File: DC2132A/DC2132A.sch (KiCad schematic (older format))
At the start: 5 parts, among them U3 LT8612

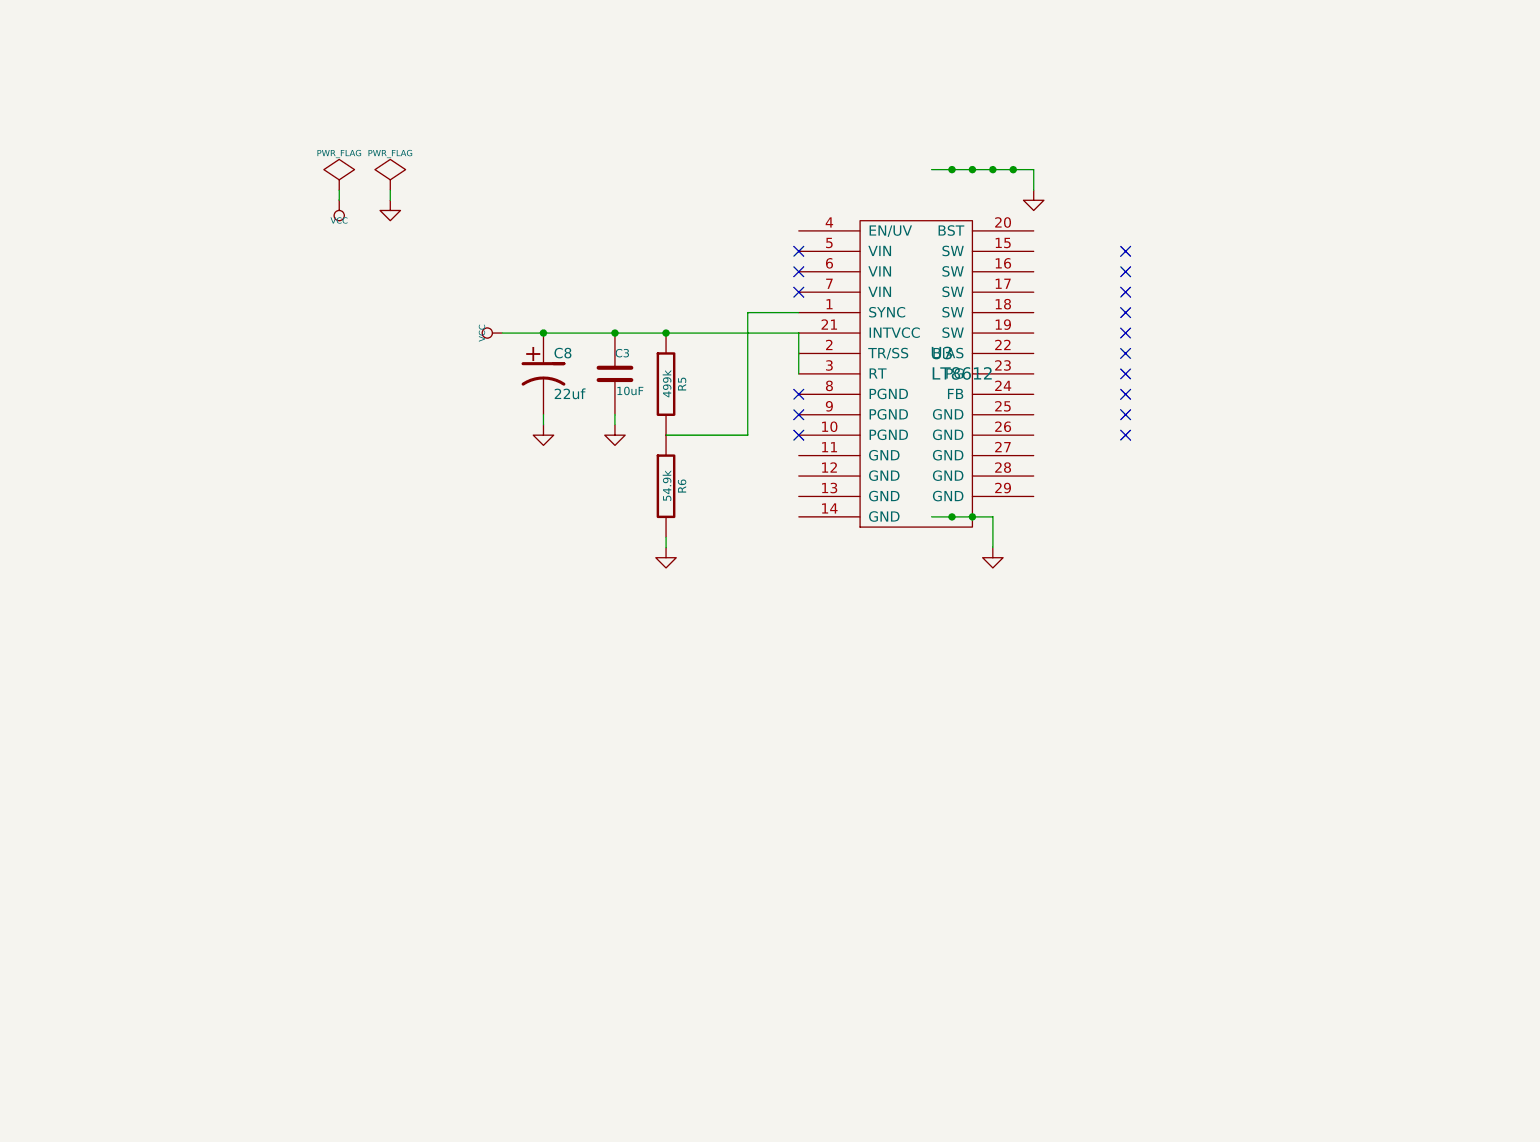
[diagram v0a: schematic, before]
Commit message: new kicad version
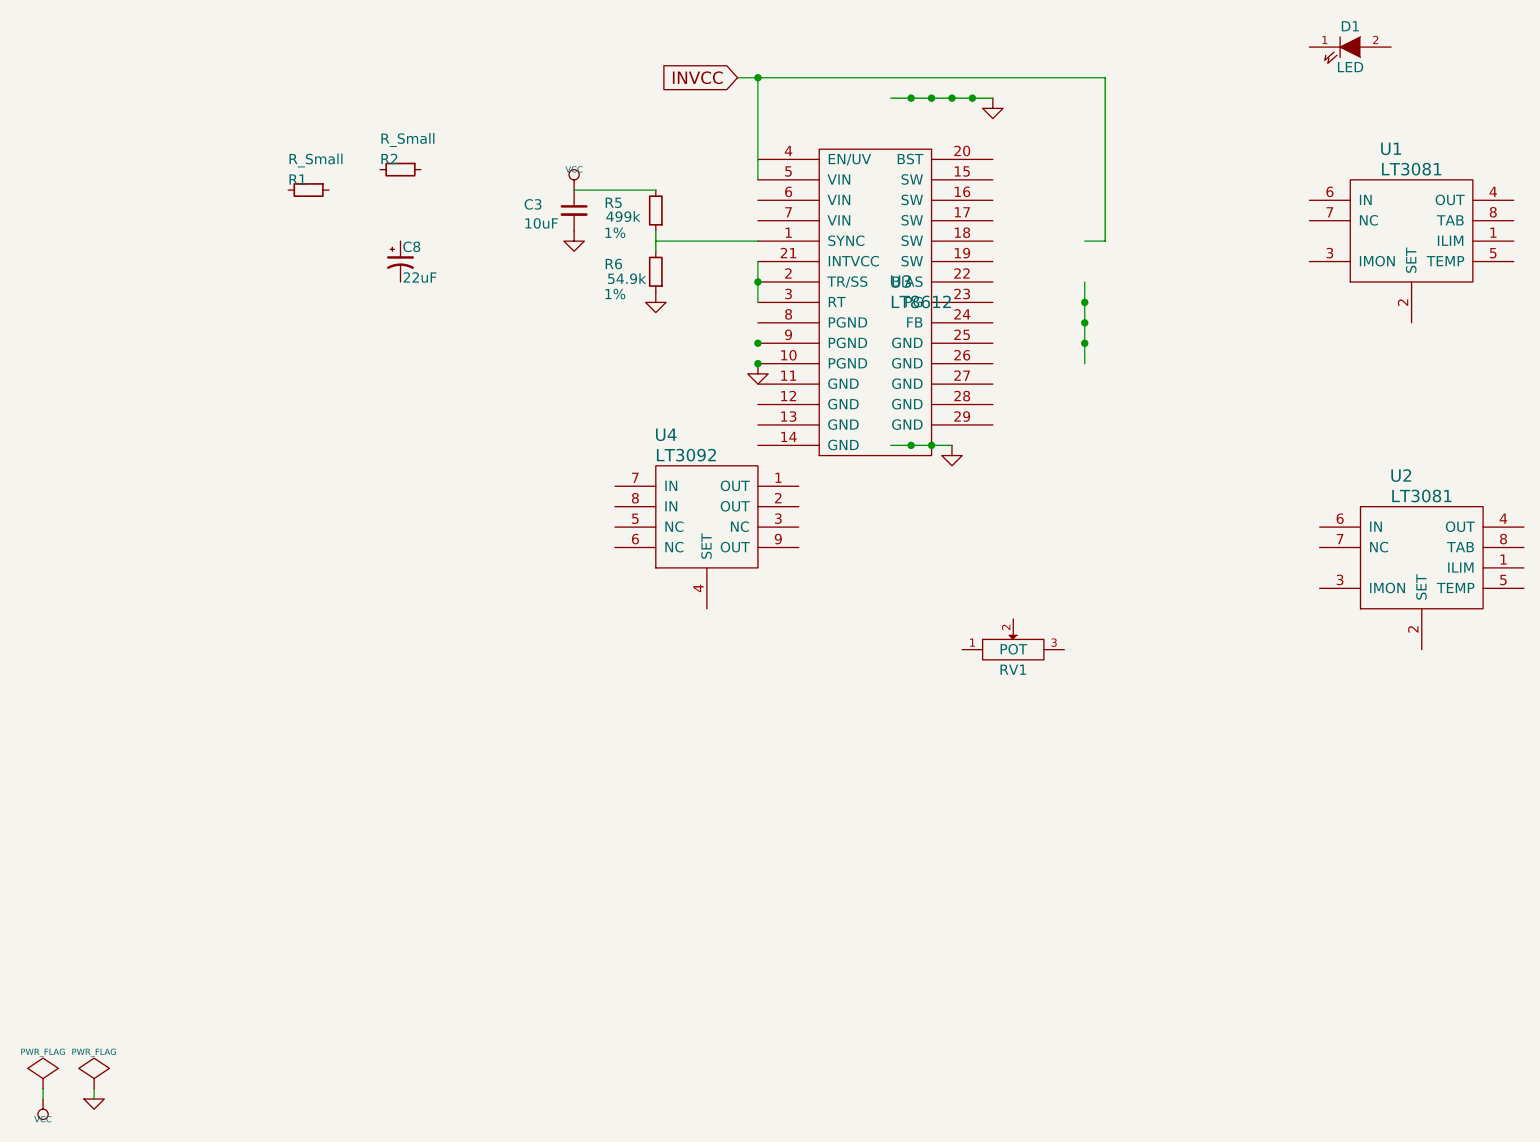
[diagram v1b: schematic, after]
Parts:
- removed C3: 10uF, ~, symbol C
- removed C8: 22uf, ~, symbol CP1
- removed R5: 499k, ~, symbol R
- removed R6: 54.9k, ~, symbol R
- added C3: 10uF, TO_SOT_Packages_SMD:TO-50-3_LongPad-NoHole_Housing, symbol C_Small
- added C8: 22uF, Power_Integrations:TO-263-7C, symbol CP1_Small
- added D1: LED, LEDs:LED-3MM, symbol LED
- added R1, R2: R_Small, Resistors_SMD:R_0603, symbol R_Small
- added R5: 499k, Resistors_SMD:R_0603, symbol R_Small
- added R6: 54.9k, Resistors_SMD:R_0603, symbol R_Small
- added RV1: POT, Potentiometers:Potentiometer_Spectrol-Type148-Type149_Single, symbol POT
- added U1, U2: LT3081, symbol LT3081
- added U4: LT3092, Housings_DFN_QFN:DFN-8-1EP_3x3mm_Pitch0.5mm, symbol LT3092
- U3: footprint ~ -> Housings_DFN_QFN:QFN-28-1EP_3x6mm_Pitch0.5mm
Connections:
- net labels added: INVCC
- wire segments 14 -> 13
- no-connect marks 16 -> 0
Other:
- moved on the sheet: U3
